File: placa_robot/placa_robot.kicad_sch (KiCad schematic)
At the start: 22 parts, among them IC1 MSP430FR2355TPT, J1 Conn_01x03, J2 Conn_01x04, J3 Conn_02x04_Odd_Even, J4 conn_DFrobot, Y1 Crystal

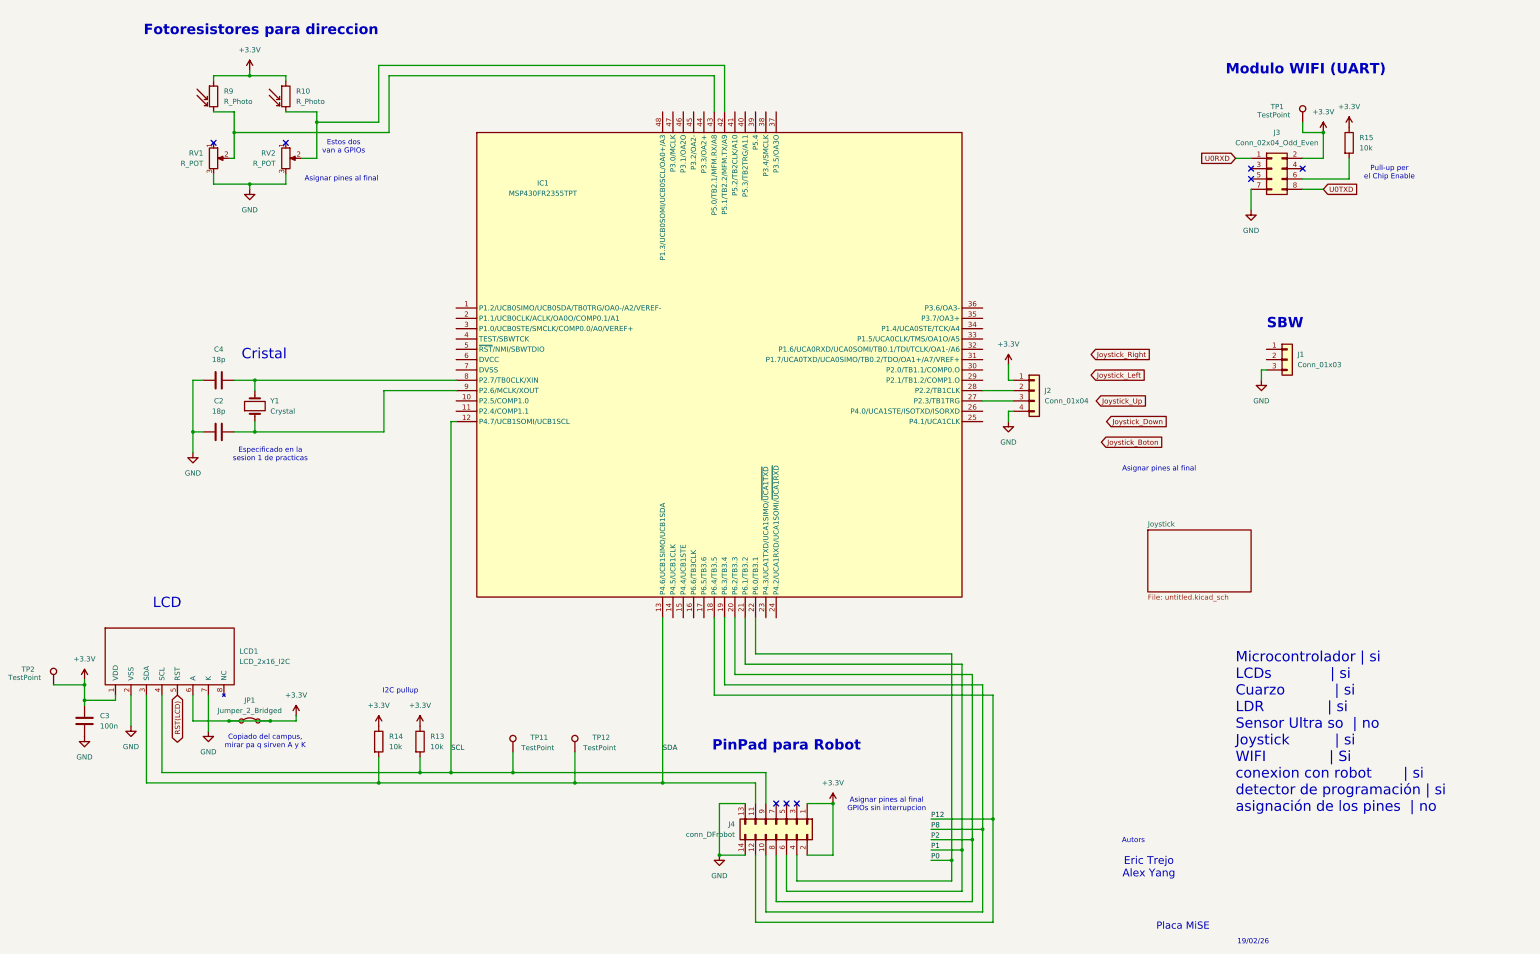
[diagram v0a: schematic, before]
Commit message: SBW reset
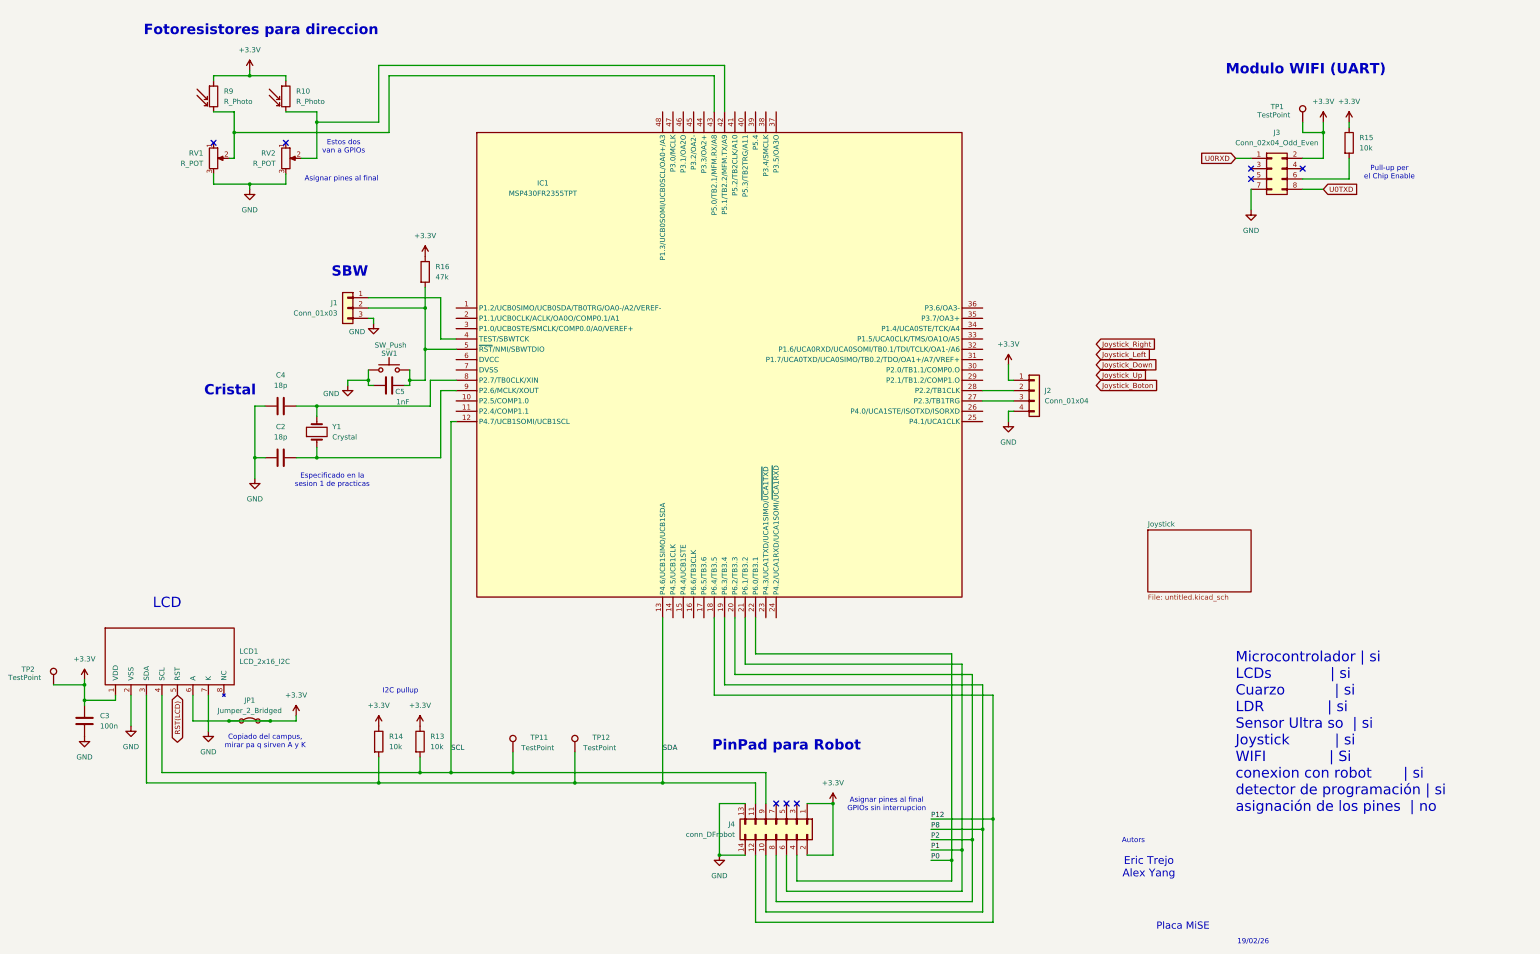
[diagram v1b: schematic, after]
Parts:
- added C5: 1nF, symbol Device:C
- added R16: 47k, symbol Device:R
- added SW1: SW_Push, symbol Switch:SW_Push
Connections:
- net +3.3V: now also R16.1
- net GND: now also C5.1, SW1.1
- net at IC1.4 (TEST/SBWTCK): now also J1.1 (Pin_1)
- net at IC1.5 (~{RST}/NMI/SBWTDIO): now also J1.2 (Pin_2), C5.2, R16.2, SW1.2
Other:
- note added: "Microcontrolador | si LCDs | si Cuarzo | si️ LDR | si Sensor Ultra so | si Joystick | si WIFI | Si conexion con robot | si detector de programación | si asignación de los pines | no"
- note removed: "Microcontrolador | si LCDs | si Cuarzo | si️ LDR | si Sensor Ultra so | no Joystick | si WIFI | Si conexion con robot | si detector de programación | si asignación de los pines | no"
- moved on the sheet: C2, C4, J1, Y1

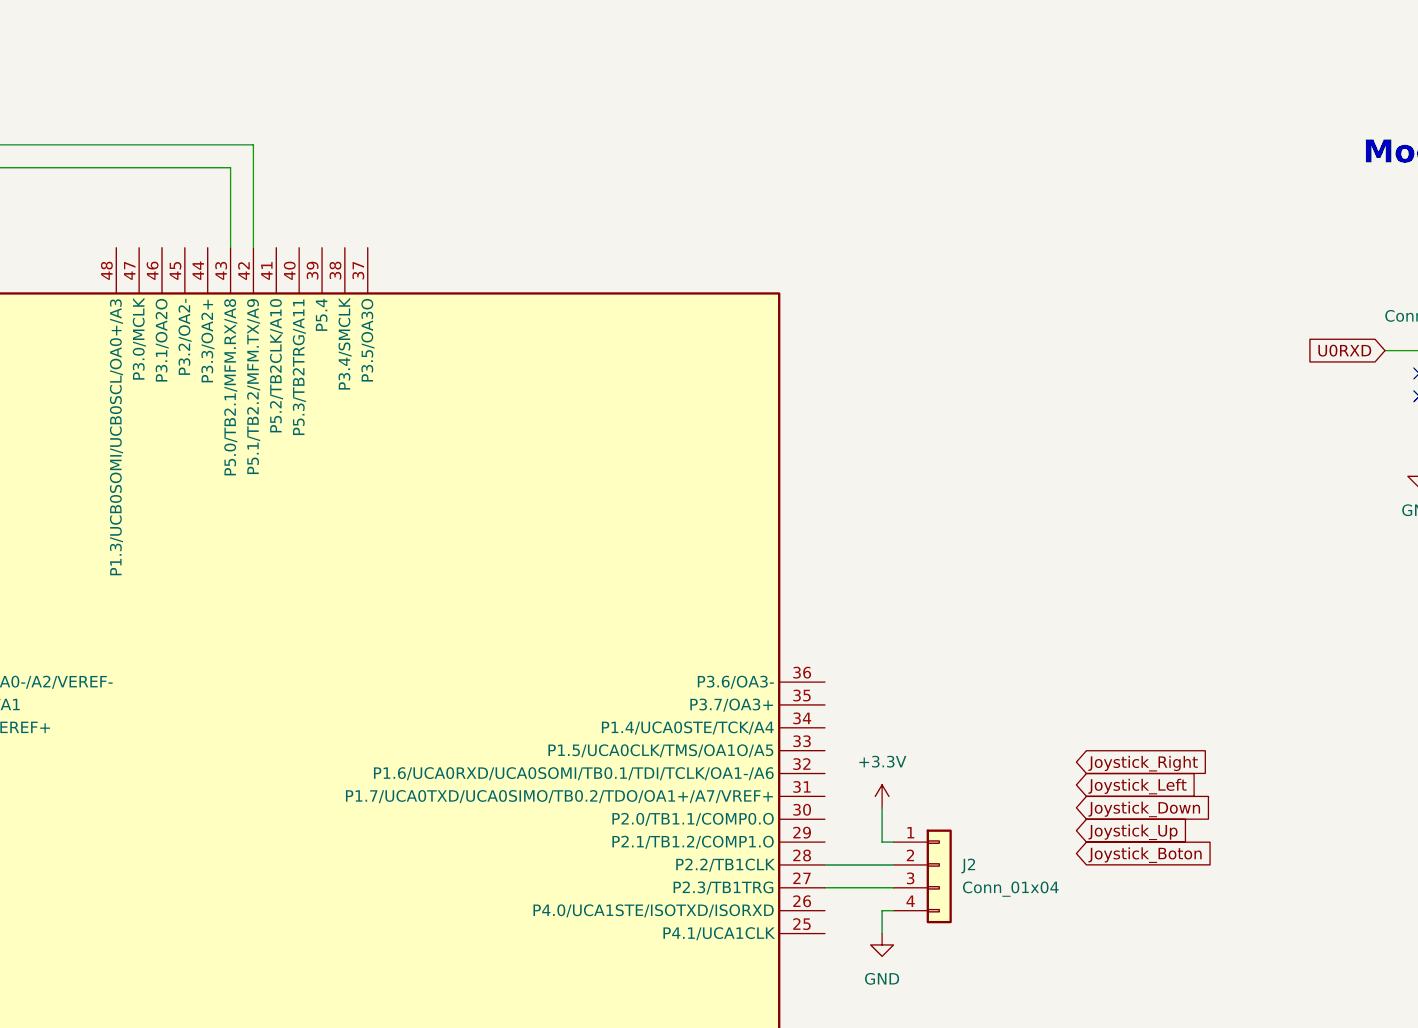
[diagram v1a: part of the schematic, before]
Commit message: Connectar Joystick
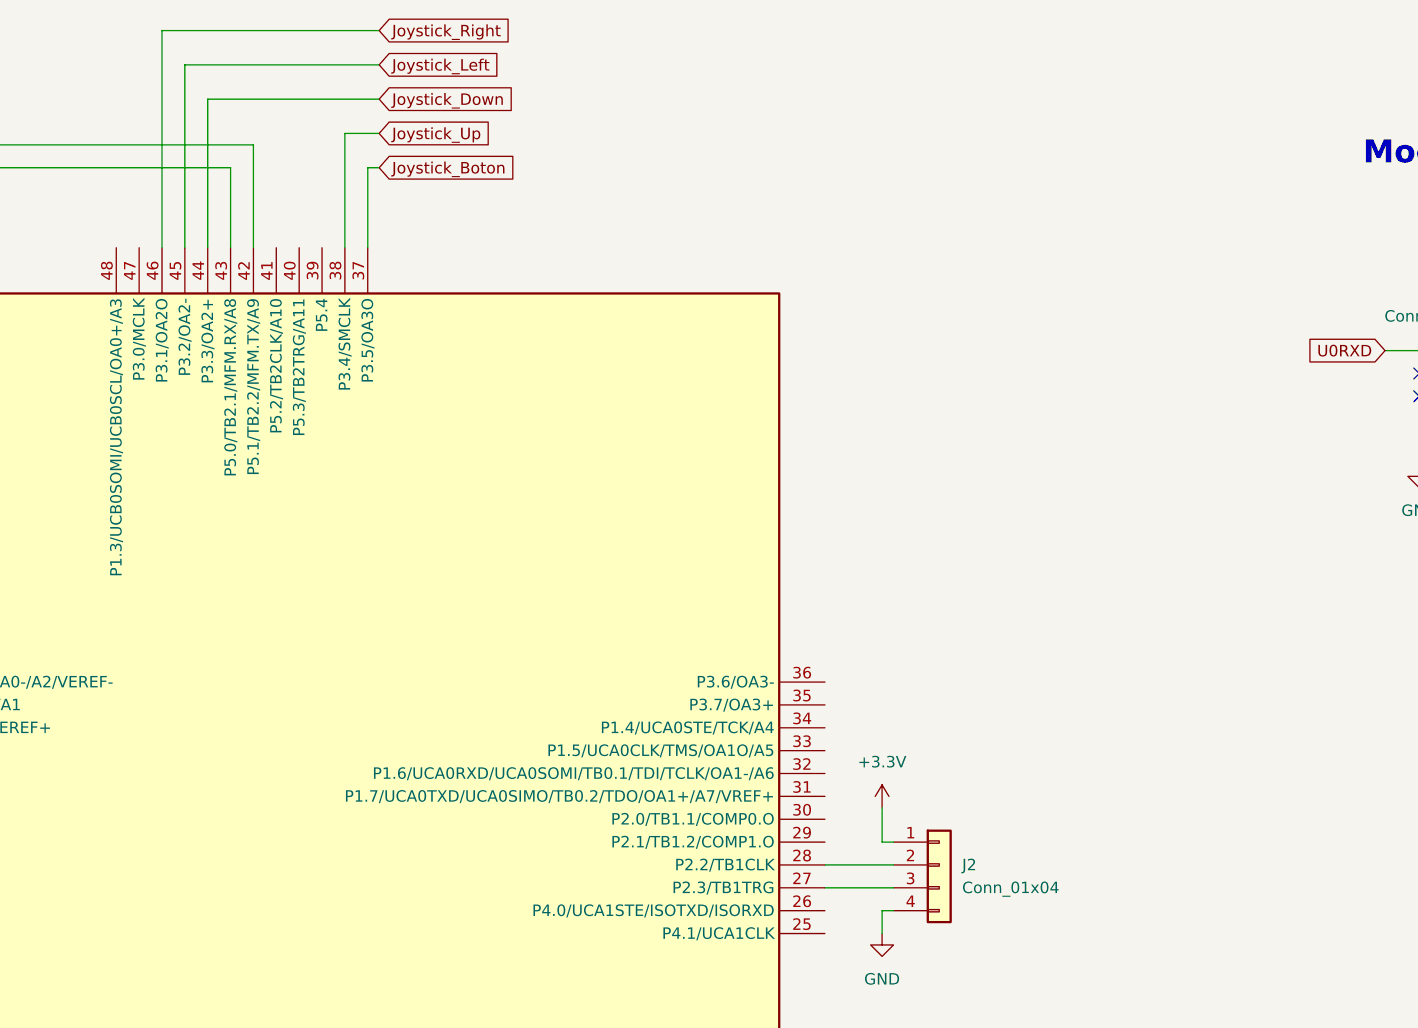
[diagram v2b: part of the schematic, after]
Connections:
- net Joystick_Boton: now also IC1.37 (P3.5/OA3O)
- net Joystick_Down: now also IC1.44 (P3.3/OA2+)
- net Joystick_Left: now also IC1.45 (P3.2/OA2-)
- net Joystick_Right: now also IC1.46 (P3.1/OA2O)
- net Joystick_Up: now also IC1.38 (P3.4/SMCLK)
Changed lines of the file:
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@@
+	(wire
+		(pts
+			(xy 199.39 59.69) (xy 199.39 76.2)
+		)
+		(stroke
+			(width 0)
+			(type default)
+		)
+	)
 	(wire
 		(pts
@@
 	(wire
 		(pts
+			(xy 214.63 63.5) (xy 214.63 76.2)
+		)
+		(stroke
+			(width 0)
+			(type default)
+		)
+	)
+	(wire
+		(pts
 			(xy 214.63 259.08) (xy 214.63 273.05)
 		)
@@
 	(wire
 		(pts
+			(xy 218.44 59.69) (xy 199.39 59.69)
+		)
+		(stroke
+			(width 0)
+			(type default)
+		)
+	)
+	(wire
+		(pts
 			(xy 274.32 152.4) (xy 274.32 149.86)
 		)
@@
 	(wire
 		(pts
+			(xy 218.44 63.5) (xy 214.63 63.5)
+		)
+		(stroke
+			(width 0)
+			(type default)
+		)
+	)
+	(wire
+		(pts
 			(xy 267.97 147.32) (xy 275.59 147.32)
 		)
@@
 	(wire
 		(pts
+			(xy 218.44 55.88) (xy 196.85 55.88)
+		)
+		(stroke
+			(width 0)
+			(type default)
+		)
+	)
+	(wire
+		(pts
 			(xy 130.81 134.62) (xy 138.43 134.62)
 		)
@@
 	(wire
 		(pts
+			(xy 196.85 55.88) (xy 196.85 76.2)
+		)
+		(stroke
+			(width 0)
+			(type default)
+		)
+	)
+	(wire
+		(pts
 			(xy 83.82 76.2) (xy 78.74 76.2)
 		)
@@
 	(wire
 		(pts
+			(xy 217.17 67.31) (xy 217.17 76.2)
+		)
+		(stroke
+			(width 0)
+			(type default)
+		)
+	)
+	(wire
+		(pts
 			(xy 54.61 220.98) (xy 54.61 219.71)
 		)
@@
 	(wire
 		(pts
+			(xy 194.31 52.07) (xy 194.31 76.2)
+		)
+		(stroke
+			(width 0)
+			(type default)
+		)
+	)
+	(wire
+		(pts
 			(xy 214.63 273.05) (xy 267.97 273.05)
 		)
@@
 	(wire
 		(pts
+			(xy 218.44 52.07) (xy 194.31 52.07)
+		)
+		(stroke
+			(width 0)
+			(type default)
+		)
+	)
+	(wire
+		(pts
 			(xy 189.23 241.3) (xy 189.23 200.66)
 		)
@@
 		(pts
 			(xy 204.47 76.2) (xy 204.47 64.77)
+		)
+		(stroke
+			(width 0)
+			(type default)
+		)
+	)
+	(wire
+		(pts
+			(xy 218.44 67.31) (xy 217.17 67.31)
 		)
 		(stroke
@@
 	(global_label "Joystick_Left"
 		(shape input)
-		(at 295.91 135.89 0)
+		(at 218.44 55.88 0)
 		(fields_autoplaced yes)
 		(effects
@@
 		)
 		(property "Intersheetrefs" "${INTERSHEET_REFS}"
-			(at 310.9904 135.89 0)
+			(at 233.5204 55.88 0)
 			(effects
 				(font
@@
 	(global_label "Joystick_Boton"
 		(shape input)
-		(at 295.91 143.51 0)
+		(at 218.44 67.31 0)
 		(fields_autoplaced yes)
 		(effects
@@
 		)
 		(property "Intersheetrefs" "${INTERSHEET_REFS}"
-			(at 312.865 143.51 0)
+			(at 235.395 67.31 0)
 			(effects
 				(font
@@
 	(global_label "Joystick_Up"
 		(shape input)
-		(at 295.91 140.97 0)
+		(at 218.44 63.5 0)
 		(fields_autoplaced yes)
 		(effects
@@
 		)
 		(property "Intersheetrefs" "${INTERSHEET_REFS}"
-			(at 309.9018 140.97 0)
+			(at 232.4318 63.5 0)
 			(effects
 				(font
@@
 	(global_label "Joystick_Right"
 		(shape input)
-		(at 295.91 133.35 0)
+		(at 218.44 52.07 0)
 		(fields_autoplaced yes)
 		(effects
@@
 		)
 		(property "Intersheetrefs" "${INTERSHEET_REFS}"
-			(at 312.3208 133.35 0)
+			(at 234.8508 52.07 0)
 			(effects
 				(font
@@
 	(global_label "Joystick_Down"
 		(shape input)
-		(at 295.91 138.43 0)
+		(at 218.44 59.69 0)
 		(fields_autoplaced yes)
 		(effects
@@
 		)
 		(property "Intersheetrefs" "${INTERSHEET_REFS}"
-			(at 312.3208 138.43 0)
+			(at 234.8508 59.69 0)
 			(effects
 				(font
